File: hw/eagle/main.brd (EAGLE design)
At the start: 49.2 x 49.5 mm, 12 parts

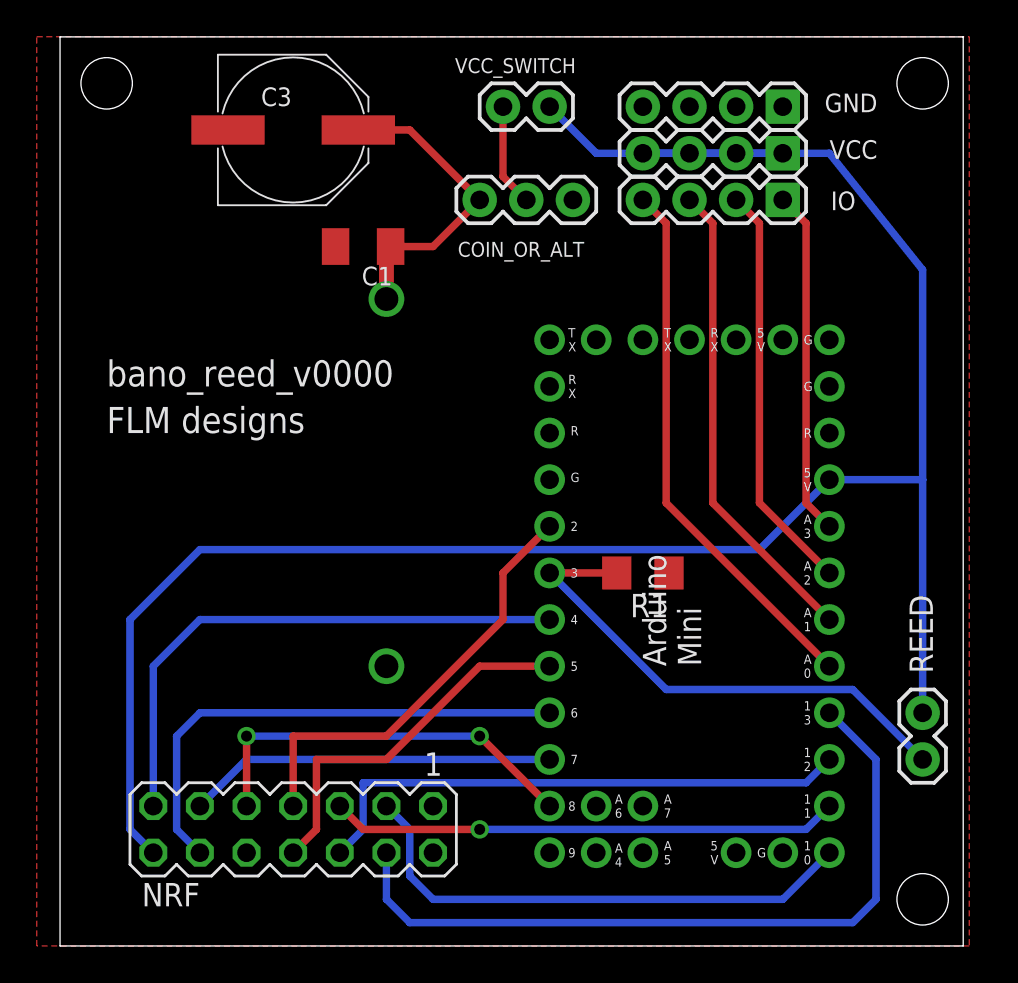
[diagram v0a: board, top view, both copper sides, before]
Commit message: [ add ] board routing, done
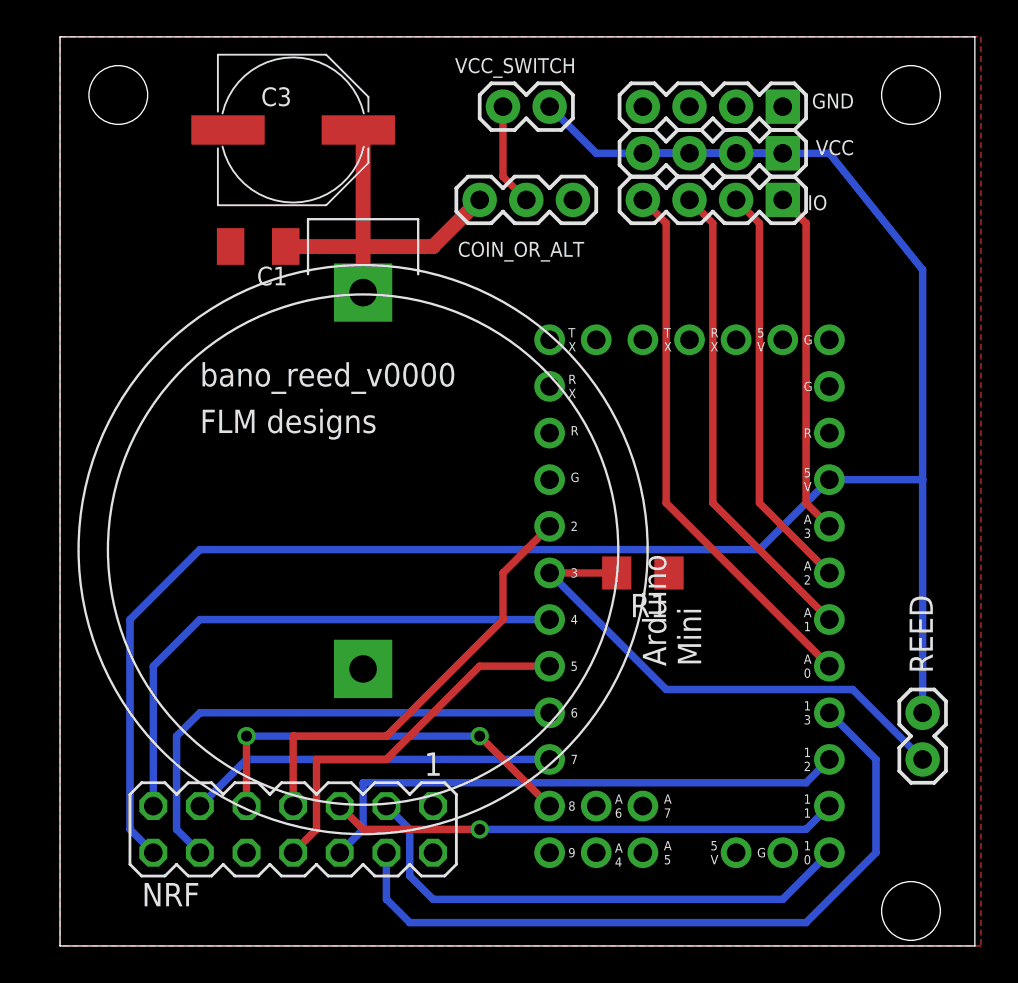
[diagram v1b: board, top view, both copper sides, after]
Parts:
- removed CON_COIN_HOLDER: (no value), SparkFun:BATTCOM_20MM_PTH
- added U$1: KEYSTONE_1025_7, keystone_1025_7:KEYSTONE_1025_7
- moved C1 5.72 mm to (10.8, 38.1)
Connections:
- net COIN_VCC: now also U$1.P$2; no longer CON_COIN_HOLDER.1
- net GND: now also U$1.P$3; no longer CON_COIN_HOLDER.2
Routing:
- net COIN_VCC: track 17.2 -> 20.7 mm
- net NRF_SCK: track 41.5 -> 40.0 mm
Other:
- board size 49.2 x 49.5 mm -> 49.8 x 49.5 mm
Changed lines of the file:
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@@
 <setting verticaltext="up"/>
 </settings>
-<grid distance="1.27" unitdist="mm" unit="mm" style="lines" multiple="1" display="yes" altdistance="0.025" altunitdist="inch" altunit="inch"/>
+<grid distance="0.635" unitdist="mm" unit="mm" style="lines" multiple="1" display="yes" altdistance="0.025" altunitdist="inch" altunit="inch"/>
 <layers>
 <layer number="1" name="Top" color="4" fill="1" visible="yes" active="yes"/>
@@
 <board>
 <plain>
-<wire x1="0" y1="0" x2="49.2" y2="0" width="0" layer="20"/>
-<wire x1="49.2" y1="0" x2="49.2" y2="49.52" width="0" layer="20"/>
-<wire x1="49.2" y1="49.52" x2="0" y2="49.52" width="0" layer="20"/>
+<wire x1="0" y1="0" x2="49.835" y2="0" width="0" layer="20"/>
+<wire x1="49.835" y1="0" x2="49.835" y2="49.52" width="0" layer="20"/>
+<wire x1="49.835" y1="49.52" x2="0" y2="49.52" width="0" layer="20"/>
 <wire x1="0" y1="49.52" x2="0" y2="0" width="0" layer="20"/>
-<hole x="2.54" y="46.99" drill="2.8"/>
-<hole x="46.99" y="46.99" drill="2.8"/>
-<hole x="46.99" y="2.54" drill="2.8"/>
-<text x="2.54" y="30.48" size="1.4224" layer="25" font="vector">bano_reed_v0000</text>
-<text x="2.54" y="27.94" size="1.4224" layer="25" font="vector">FLM designs</text>
+<hole x="3.175" y="46.355" drill="3.2"/>
+<hole x="46.355" y="46.355" drill="3.2"/>
+<hole x="46.355" y="1.905" drill="3.2"/>
+<text x="7.62" y="30.48" size="1.27" layer="25" font="vector">bano_reed_v0000</text>
+<text x="7.62" y="27.94" size="1.27" layer="25" font="vector">FLM designs</text>
 </plain>
 <attributes>
@@
 <attribute name="VALUE" x="15.24" y="10.541" size="1.27" layer="27" ratio="10" rot="R180"/>
 </element>
-<element name="C1" library="rcl" package="C1206K" value="100n" x="16.51" y="38.1" rot="R180"/>
+<element name="C1" library="rcl" package="C1206K" value="100n" x="10.795" y="38.1" rot="R180"/>
 <element name="R1" library="resistor" package="R1206" value="1M" x="31.75" y="20.32" rot="R180"/>
 <element name="REED" library="SparkFun" package="1X02" value="" x="46.99" y="12.7" smashed="yes" rot="R270">
@@
 </element>
 <element name="GND" library="SparkFun" package="1X04" value="" x="39.37" y="45.72" smashed="yes" rot="R180">
-<attribute name="NAME" x="44.5262" y="46.4312" size="1.016" layer="25" ratio="10" rot="R180"/>
+<attribute name="NAME" x="43.2562" y="46.4312" size="0.8128" layer="25" ratio="10" rot="R180"/>
 <attribute name="VALUE" x="40.64" y="48.895" size="1.27" layer="27" rot="R180"/>
 </element>
 <element name="VCC" library="SparkFun" package="1X04" value="" x="39.37" y="43.18" smashed="yes" rot="R180">
-<attribute name="NAME" x="44.5262" y="43.8912" size="1.016" layer="25" ratio="10" rot="R180"/>
+<attribute name="NAME" x="43.2562" y="43.8912" size="0.8128" layer="25" ratio="10" rot="R180"/>
 <attribute name="VALUE" x="40.64" y="46.355" size="1.27" layer="27" rot="R180"/>
 </element>
 <element name="IO" library="SparkFun" package="1X04" value="" x="39.37" y="40.64" smashed="yes" rot="R180">
-<attribute name="NAME" x="41.9862" y="40.0812" size="1.016" layer="25" ratio="10" rot="R180" align="top-right"/>
+<attribute name="NAME" x="40.7162" y="40.0812" size="0.8128" layer="25" ratio="10" rot="R180" align="top-right"/>
 <attribute name="VALUE" x="40.64" y="43.815" size="1.27" layer="27" rot="R180"/>
 </element>
@@
 </element>
 <element name="C3" library="rcl" package="PANASONIC_F" value="330u" x="12.7" y="44.45"/>
-<element name="CON_COIN_HOLDER" library="SparkFun" package="BATTCOM_20MM_PTH" value="" x="17.78" y="15.24" smashed="yes" rot="MR90">
-<attribute name="NAME" x="27.305" y="15.875" size="0.4064" layer="26" rot="MR90"/>
-<attribute name="VALUE" x="17.145" y="8.255" size="0.4064" layer="28" rot="MR90"/>
-</element>
+<element name="U$1" library="keystone_1025_7" package="KEYSTONE_1025_7" value="KEYSTONE_1025_7" x="16.51" y="21.59" rot="R180"/>
 </elements>
 <signals>
@@
 <contactref element="NRF" pad="4"/>
 <contactref element="PCB1" pad="13"/>
-<wire x1="41.91" y1="12.7" x2="44.45" y2="10.16" width="0.4064" layer="16"/>
-<wire x1="44.45" y1="10.16" x2="44.45" y2="2.54" width="0.4064" layer="16"/>
-<wire x1="44.45" y1="2.54" x2="43.18" y2="1.27" width="0.4064" layer="16"/>
-<wire x1="43.18" y1="1.27" x2="19.05" y2="1.27" width="0.4064" layer="16"/>
+<wire x1="44.45" y1="10.16" x2="44.45" y2="5.08" width="0.4064" layer="16"/>
+<wire x1="44.45" y1="5.08" x2="40.64" y2="1.27" width="0.4064" layer="16"/>
+<wire x1="40.64" y1="1.27" x2="19.05" y2="1.27" width="0.4064" layer="16"/>
 <wire x1="19.05" y1="1.27" x2="17.78" y2="2.54" width="0.4064" layer="16"/>
 <wire x1="17.78" y1="2.54" x2="17.78" y2="5.08" width="0.4064" layer="16"/>
+<wire x1="41.91" y1="12.7" x2="44.45" y2="10.16" width="0.4064" layer="16"/>
 </signal>
 <signal name="GND">
@@
 <contactref element="GND" pad="1"/>
 <contactref element="C1" pad="2"/>
-<polygon width="0.4064" layer="1">
-<vertex x="-1.27" y="49.53"/>
-<vertex x="49.53" y="49.53"/>
-<vertex x="49.53" y="0"/>
-<vertex x="-1.27" y="0"/>
+<polygon width="0.4064" layer="1" isolate="0.4064">
+<vertex x="0" y="49.53"/>
+<vertex x="50.165" y="49.53"/>
+<vertex x="50.165" y="0"/>
+<vertex x="0" y="0"/>
 </polygon>
 <contactref element="C3" pad="-"/>
-<contactref element="CON_COIN_HOLDER" pad="2"/>
 <contactref element="GND" pad="2"/>
+<contactref element="U$1" pad="P$3"/>
 </signal>
 <signal name="NRF_MISO">
@@
 <contactref element="C1" pad="1"/>
 <contactref element="C3" pad="+"/>
-<contactref element="CON_COIN_HOLDER" pad="1"/>
-<wire x1="22.86" y1="40.64" x2="19.05" y2="44.45" width="0.4064" layer="1"/>
-<wire x1="19.05" y1="44.45" x2="16.25" y2="44.45" width="0.4064" layer="1"/>
-<wire x1="18.01" y1="38.1" x2="20.32" y2="38.1" width="0.4064" layer="1"/>
-<wire x1="20.32" y1="38.1" x2="22.86" y2="40.64" width="0.4064" layer="1"/>
-<wire x1="17.78" y1="35.24" x2="17.78" y2="38.1" width="0.8128" layer="1"/>
-<wire x1="17.78" y1="38.1" x2="18.01" y2="38.1" width="0.4064" layer="1"/>
+<wire x1="16.51" y1="38.1" x2="20.32" y2="38.1" width="0.8128" layer="1"/>
+<wire x1="20.32" y1="38.1" x2="22.86" y2="40.64" width="0.8128" layer="1"/>
+<contactref element="U$1" pad="P$2"/>
+<wire x1="16.51" y1="38.1" x2="12.295" y2="38.1" width="0.8128" layer="1"/>
+<wire x1="16.51" y1="35.59" x2="16.51" y2="38.1" width="0.8128" layer="1"/>
+<wire x1="16.51" y1="38.1" x2="16.51" y2="44.45" width="0.8128" layer="1"/>
+<wire x1="16.51" y1="44.45" x2="16.25" y2="44.45" width="0.4064" layer="1"/>
 </signal>
 <signal name="ALT_VCC">
